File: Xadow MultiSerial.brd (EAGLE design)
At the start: 25.4 x 20.3 mm, 45 parts, among them J1 12p 0.5mm bottom contact, J2 12p 0.5mm bottom contact, J3 12p 0.5mm bottom contact, J4 12p 0.5mm bottom contact, Q1 MOSFET-N-044020001, Q2 MOSFET-N-044020001, Q3 MOSFET-N-044020001, Q4 MOSFET-N-044020001, Q5 MOSFET-N-044020001, Q6 MOSFET-N-044020001, U1 SC16IS752, X1 CTS_32X25_SMD

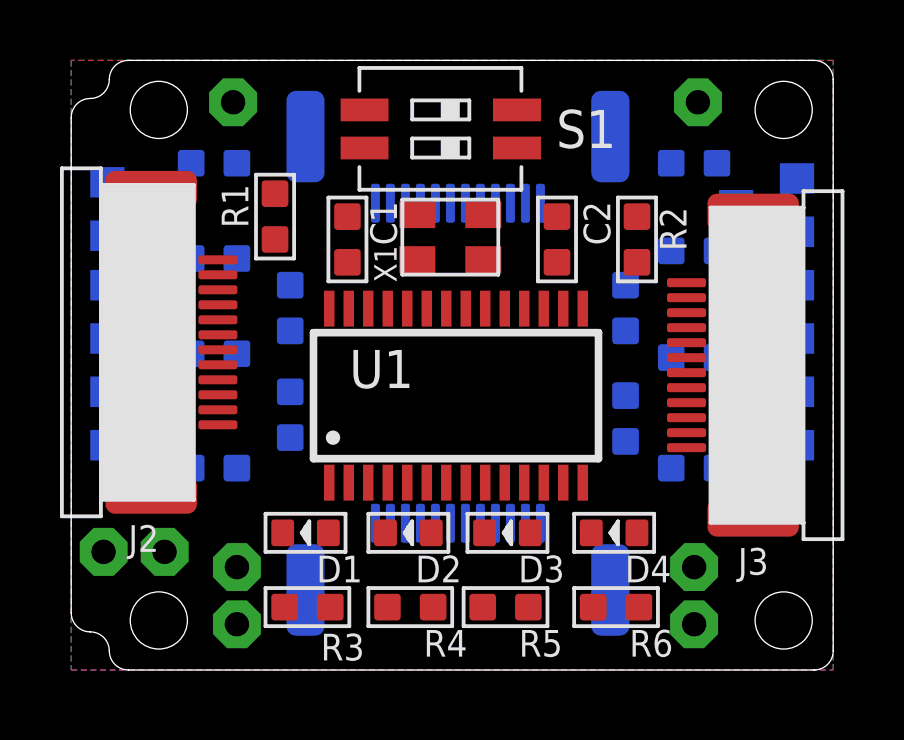
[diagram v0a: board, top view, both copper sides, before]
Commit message: Fixed errors and relayed out, last attempt with MOSFET level shifter, need to try TXS shifter
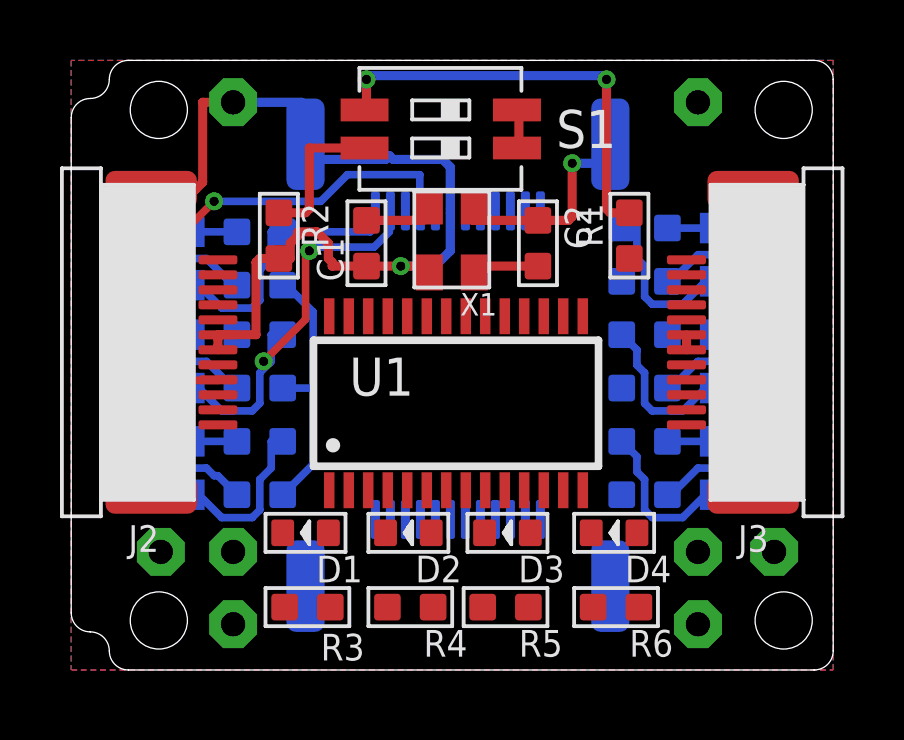
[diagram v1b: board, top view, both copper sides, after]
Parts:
- moved RXA_5 20.3 mm to (25.5, 4.95)
- moved TXB_5 15.4 mm to (7.49, 4.95)
- moved TXO_5 15.4 mm to (23.0, 4.95)
- moved RXB_5 15.4 mm to (7.49, 2.54)
- moved RXI_5 15.4 mm to (23.0, 2.54)
- moved R2 11.9 mm to (9.02, 15.5)
- moved R1 11.8 mm to (20.7, 15.5)
- moved R12 6.31 mm to (8.38, 6.86), turned to 180 degrees
- moved R18 6.26 mm to (21.2, 6.86), turned to 0 degrees
- moved R8 4.34 mm to (8.38, 13.8)
- moved R14 4.27 mm to (21.2, 14.0), turned to 0 degrees
- moved R16 3.14 mm to (21.2, 10.4), turned to 0 degrees
- moved R10 3.07 mm to (8.38, 10.4)
- moved TXA_5 1.91 mm to (5.08, 4.95)
- moved R15 1.82 mm to (21.2, 12.2), turned to 0 degrees
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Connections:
- net N$3: no longer R2.2
- net N$5: now also R2.2
- net PB1/D15/SCK: now also J4.1; no longer J4.12
- net PB2/D16/MOSI: now also J4.2; no longer J4.11
- net PB3/D14/MISO: now also J4.3; no longer J4.10
- net PD0/SCL/D3: now also J4.9; no longer J4.4
- net PD1/SDA/D2: now also J4.10; no longer J4.3
- net PF0/A5: now also J4.4; no longer J4.9
- net RXA: now also J4.11; no longer J4.2
- net TXA: now also J4.12; no longer J4.1
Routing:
- net GND: track 0.00 -> 40.3 mm, vias 0 -> 2
- net 3V3: track 0.00 -> 22.7 mm
- net PD0/SCL/D3: track 0.00 -> 16.1 mm, vias 0 -> 1
- net N$3: track 0.00 -> 14.3 mm, vias 0 -> 2
- net RXB: track 0.00 -> 13.9 mm, vias 0 -> 2
- net TXB: track 0.00 -> 9.34 mm
- net N$17: track 0.00 -> 8.92 mm
- net TXA: track 0.00 -> 5.66 mm
- net N$5: track 0.00 -> 4.94 mm
- net N$19: track 0.00 -> 4.05 mm
- net N$22: track 0.00 -> 4.05 mm
- net N$20: track 0.00 -> 4.05 mm
- net N$23: track 0.00 -> 4.05 mm
- net N$21: track 0.00 -> 4.05 mm
- net N$18: track 0.00 -> 4.05 mm
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
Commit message: Added TXS based level translation
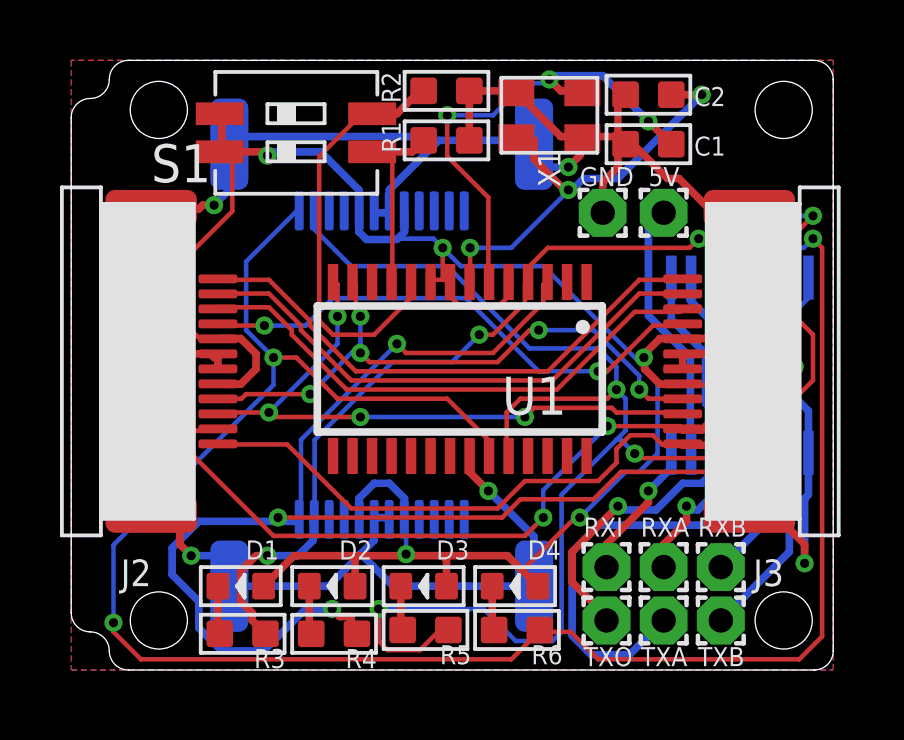
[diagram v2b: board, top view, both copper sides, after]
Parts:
- removed Q1, Q2, Q3, Q4, Q5, Q6: MOSFET-N-044020001, OPL:SOT23
- removed R10, R11, R12, R13, R14, R15, R16, R17, R18, R7, R8, R9: 10K, OPL:R0603
- removed RXA_5, RXB_5, RXI_5, TXA_5, TXB_5, TXO_5: WIREPAD1,6/0,8, wirepad:1,6/0,8
- added RXA, RXB, RXI, TXA, TXB, TXO: (no value), wirepad:1,6/0,8
- added U2: TXB0106PWR, Texas Instruments_By_element14_Batch_1:SOP65P640X120-16N
- 5V, GND: value WIREPAD1,6/0,8 -> (none)
- moved GND 12.9 mm to (19.8, 16.3), flipped to the top
- moved C1 9.96 mm to (21.3, 18.5), turned to 0 degrees
- moved R2 7.38 mm to (14.6, 20.3), turned to 180 degrees
- moved R1 6.87 mm to (14.6, 18.7), turned to 180 degrees
- moved C2 6.17 mm to (21.3, 20.2), turned to 0 degrees
- moved X1 5.34 mm to (18.0, 19.6), turned to 180 degrees
- moved S1 4.96 mm to (9.59, 19.6), turned to 270 degrees
- moved 5V 3.86 mm to (21.8, 16.3), flipped to the top
- moved D4 3.75 mm to (16.9, 3.81)
- moved R6 3.39 mm to (17.0, 2.35)
- moved D3 3.31 mm to (13.8, 3.81)
- moved D2 3.10 mm to (10.8, 3.81)
- moved D1 2.80 mm to (7.75, 3.81)
- moved R5 2.77 mm to (13.9, 2.35)
- moved R4 2.69 mm to (10.9, 2.22)
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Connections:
- removed net N$17: 5V.1, R10.2, R12.2, R14.2, R16.2, R18.2, R8.2
- new net N$4: 5V.1, U2.15
- net 3V3: now also U2.2, U2.8; no longer Q1.1, Q2.1, Q3.1, Q4.1, Q5.1, Q6.1, R11.2, R13.2, R15.2, R17.2, R7.2, R9.2
- net GND: now also U2.9
- net N$18: now also RXI.1, U2.16; no longer Q1.3, R8.1, TXB_5.1
- net N$19: now also TXO.1, U2.14; no longer Q2.3, R10.1, RXB_5.1
- net N$20: now also RXA.1, U2.13; no longer Q3.3, R12.1, TXA_5.1
- net N$21: now also TXA.1, U2.12; no longer Q4.3, R14.1, RXA_5.1
- net N$22: now also RXB.1, U2.11; no longer Q5.3, R16.1, TXO_5.1
- net N$23: now also TXB.1, U2.10; no longer Q6.3, R18.1, RXI_5.1
- net PB1/D15/SCK: no longer J1.12, J4.1
- net PB2/D16/MOSI: no longer J1.11, J4.2
- net PB3/D14/MISO: no longer J1.10, J4.3
- net PD0/SCL/D3: no longer J1.4, J4.9
- net PD1/SDA/D2: no longer J1.3, J4.10
- net PD2/RXI/D0: now also U2.1; no longer Q6.2, R17.1
- net PD3/TXO/D1: now also U2.3; no longer Q5.2, R15.1
- net PF0/A5: no longer J1.9, J4.4
- net RXA: now also U2.4; no longer Q4.2, R13.1
- net RXB: now also U2.6; no longer Q2.2, R9.1
- net TXA: now also U2.5; no longer Q3.2, R11.1
- net TXB: now also U2.7; no longer Q1.2, R7.1
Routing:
- net TXB: track 9.34 -> 66.5 mm, vias 0 -> 3
- net 3V3: track 22.7 -> 76.3 mm, vias 0 -> 7
- net TXA: track 5.66 -> 57.5 mm, vias 0 -> 4
- net GND: track 40.3 -> 88.8 mm, vias 2 -> 6
- net RXB: track 13.9 -> 49.7 mm, vias 2 -> 4
- net PD2/RXI/D0: track 1.65 -> 27.8 mm, vias 0 -> 3
- net RXA: track 1.65 -> 26.9 mm, vias 0 -> 3
- net PD3/TXO/D1: track 1.65 -> 25.8 mm, vias 0 -> 1
- net PD1/SDA/D2: track 0.00 -> 21.2 mm, vias 0 -> 4
- net PB1/D15/SCK: track 0.00 -> 18.1 mm
- net PB2/D16/MOSI: track 0.00 -> 18.0 mm
- net PB3/D14/MISO: track 0.00 -> 17.9 mm
- net PF0/A5: track 0.00 -> 17.6 mm, vias 0 -> 2
- net N$1: track 2.26 -> 16.5 mm, vias 0 -> 3
- net N$2: track 2.21 -> 14.9 mm, vias 0 -> 3
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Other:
- board text added: "by Tisham Dhar"
- board text removed: "by Seeed Studio"
